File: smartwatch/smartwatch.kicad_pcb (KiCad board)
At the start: 4 copper layers, 40.1 x 40.1 mm, 32 parts, among them J1 BAT_CON, J2 DC_CON, J3 PROG_INT, J4 I2C Touch, J5 SPI Display, J6 Power, J7 Micro_SD_Card, SW1 SW_Push, U1 ESP32-WROVER-E, U2 MCP73831-5-OT, U3 MPU-6050, U4 TLV1117-33

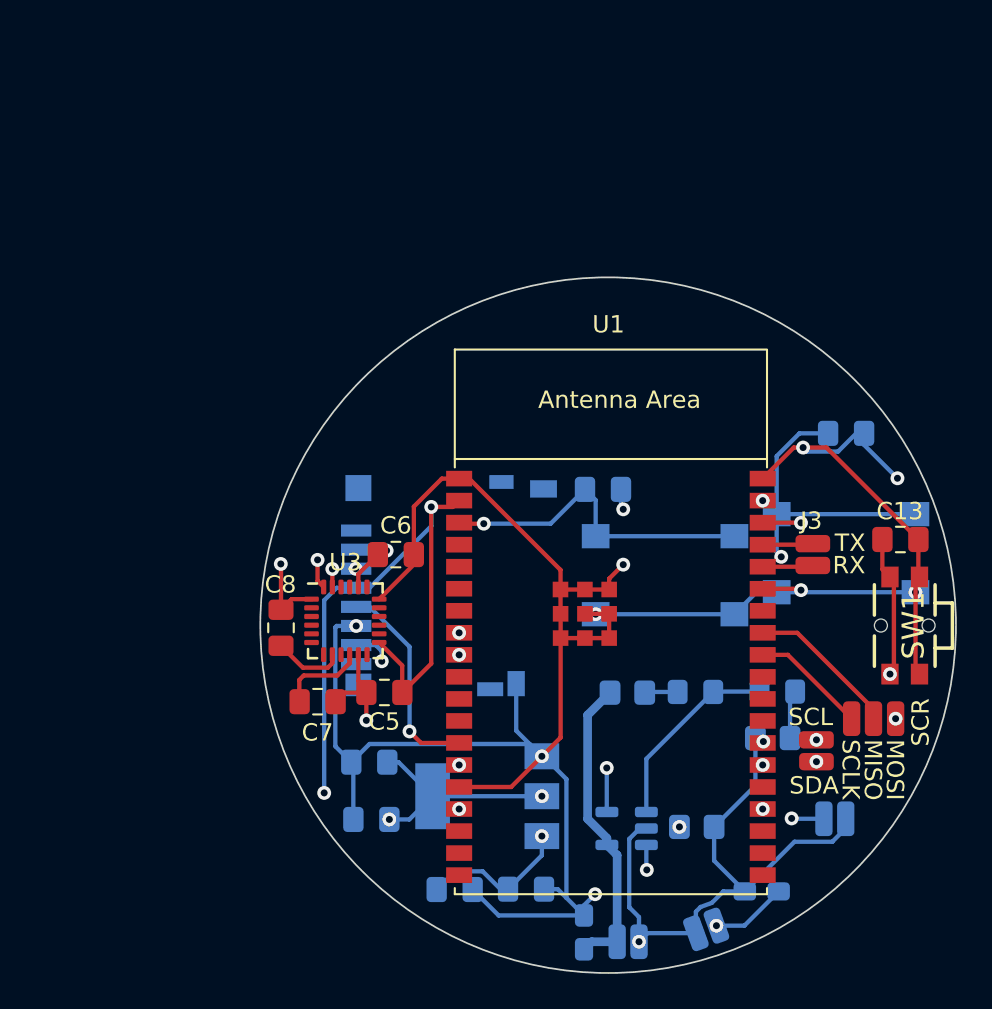
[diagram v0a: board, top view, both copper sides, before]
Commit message: updated pcb schematic and design
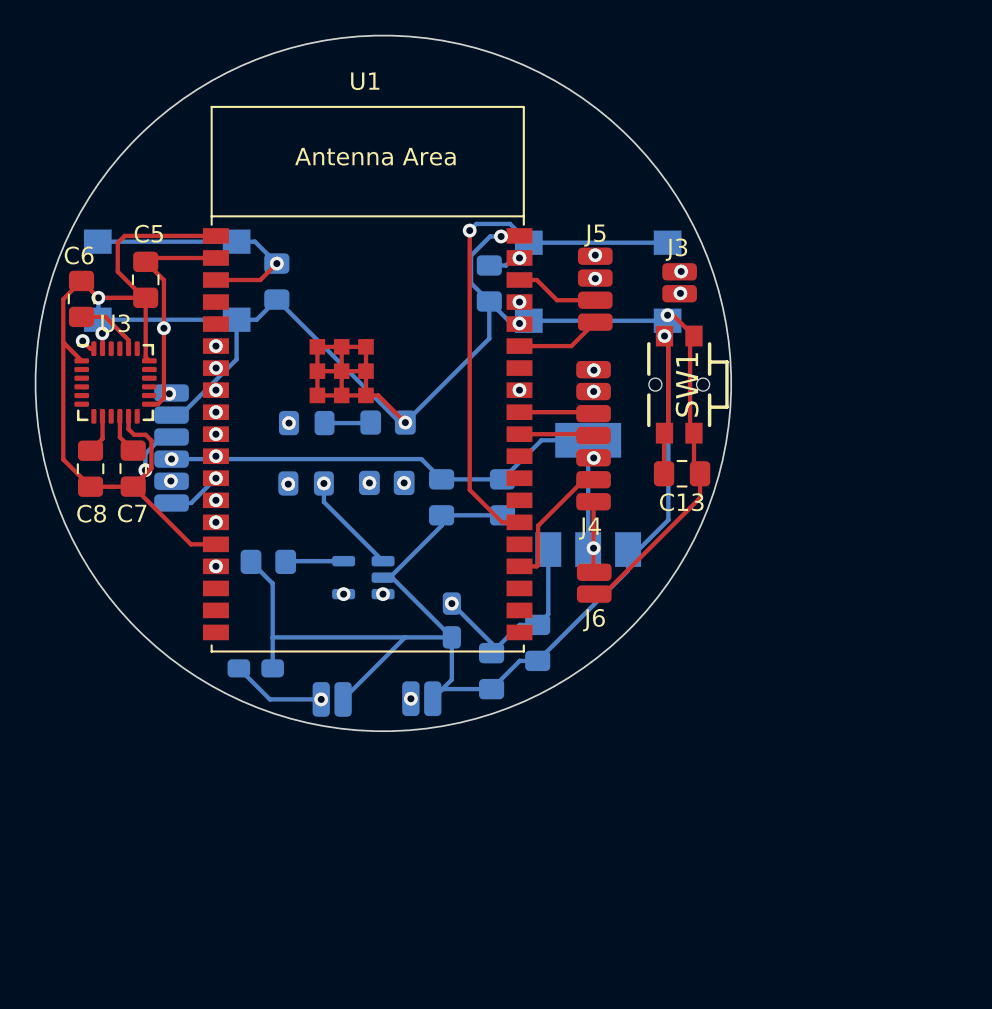
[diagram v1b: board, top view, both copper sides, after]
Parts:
- removed J7: Micro_SD_Card, Connector_Card:microSD_HC_Hirose_DM3D-SF
- added J8: SD Card, Connector_Wire_SMD:Wire_Pad_1x06, B.Cu at (33.3, 46.2)
- J4: value I2C Touch -> Screen; footprint Connector_Wire_SMD:Wire_Pad_1x02 -> Connector_Wire_SMD:Wire_Pad_1x07
- J5: value SPI Display -> Touch; footprint Connector_Wire_SMD:Wire_Pad_1x03 -> Connector_Wire_SMD:Wire_Pad_1x04
- J6: moved to F.Cu
- moved RST1 33.3 mm to (33.1, 36.5)
- moved GREEN1 31.2 mm to (41.1, 44.8)
- moved J5 29.5 mm to (57.7, 37.0), turned to -90 degrees
- moved R1 29.0 mm to (38.9, 52.8), turned to 180 degrees
- moved R3 28.7 mm to (45.8, 44.7), turned to 0 degrees
- moved C5 27.5 mm to (31.8, 36.5), turned to -90 degrees
- moved RED1 25.5 mm to (41.1, 48.2)
- moved C12 24.3 mm to (38.2, 58.9), turned to 0 degrees
- moved C11 23.7 mm to (49.5, 56.1), turned to -90 degrees
- moved C6 23.4 mm to (28.1, 37.6), turned to 90 degrees
- moved C9 22.3 mm to (51.6, 36.7), turned to 90 degrees
- moved C10 22.3 mm to (39.4, 36.6), turned to 90 degrees
- moved J4 22.2 mm to (57.6, 45.5)
- moved J2 22.1 mm to (42.6, 60.7)
- moved BOOT/FLASH1 21.2 mm to (57.9, 36.6)
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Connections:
- J4 pad 1: TOUCH_SCL -> SCR_MISO
- J4 pad 2: TOUCH_SDA -> SCR_MOSI
- J5 pad 1: SCR_SCLK -> TOUCH_RST
- J5 pad 2: SCR_MISO -> TOUCH_IRQ
- J5 pad 3: SCR_MOSI -> TOUCH_SCL
- U1 pad 10: unconnected-(U1-DAC_1/ADC2_CH8/GPIO25-Pad10) -> TOUCH_IRQ
- U1 pad 11: unconnected-(U1-DAC_2/ADC2_CH9/GPIO26-Pad11) -> TOUCH_RST
- U1 pad 12: unconnected-(U1-ADC2_CH7/GPIO27-Pad12) -> SD_SS
- U1 pad 23: SD_SS -> SCR_RST
- U1 pad 26: BTN_INP -> unconnected-(U1-ADC2_CH0/GPIO4-Pad26)
- U1 pad 29: unconnected-(U1-GPIO5-Pad29) -> SCR_CS
- U1 pad 31: SCR_MISO -> SCR_DC
- U1 pad 6: unconnected-(U1-GPIO34/ADC1_CH6-Pad6) -> BTN_INP
- U1 pad 7: unconnected-(U1-GPIO35/ADC1_CH7-Pad7) -> SCR_MISO
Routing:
- net TOUCH_RST: track 0.00 -> 27.2 mm, vias 0 -> 2
- net SD_SS: track 29.6 -> 3.15 mm, vias 2 -> 1
- net TOUCH_IRQ: track 0.00 -> 25.6 mm, vias 0 -> 3
- net BTN_INP: track 17.1 -> 34.2 mm
- net 3V3: track 71.5 -> 57.3 mm, vias 5 -> 3
- net SCR_MISO: track 8.76 -> 21.9 mm, vias 0 -> 2
- net SD_MOSI: track 16.7 -> 6.04 mm
- net TOUCH_SCL: track 15.5 -> 4.85 mm, vias 2 -> 0
- net SCR_RST: track 0.00 -> 7.67 mm
- net TOUCH_SDA: track 12.5 -> 4.94 mm, vias 2 -> 0
- net SCR_MOSI: track 17.3 -> 10.0 mm
- net TX: track 2.91 -> 10.1 mm, vias 0 -> 2
- net RX: track 2.92 -> 10.1 mm, vias 0 -> 2
- net SCR_DC: track 0.00 -> 5.91 mm, vias 0 -> 2
- net BAT_VDD: track 26.9 -> 21.5 mm
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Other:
- board text removed: "3V3"
- board text removed: "DCIN"
- board text removed: "GND"
- board text removed: "MISO"
- board text removed: "MOSI"
- board text removed: "RX"
- board text removed: "SCL"
- board text removed: "SCLK"
- board text removed: "SCR"
- board text removed: "SDA"
- board text removed: "TX"
- board text removed: "VDD"
